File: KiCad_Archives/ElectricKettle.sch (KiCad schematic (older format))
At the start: 11 parts

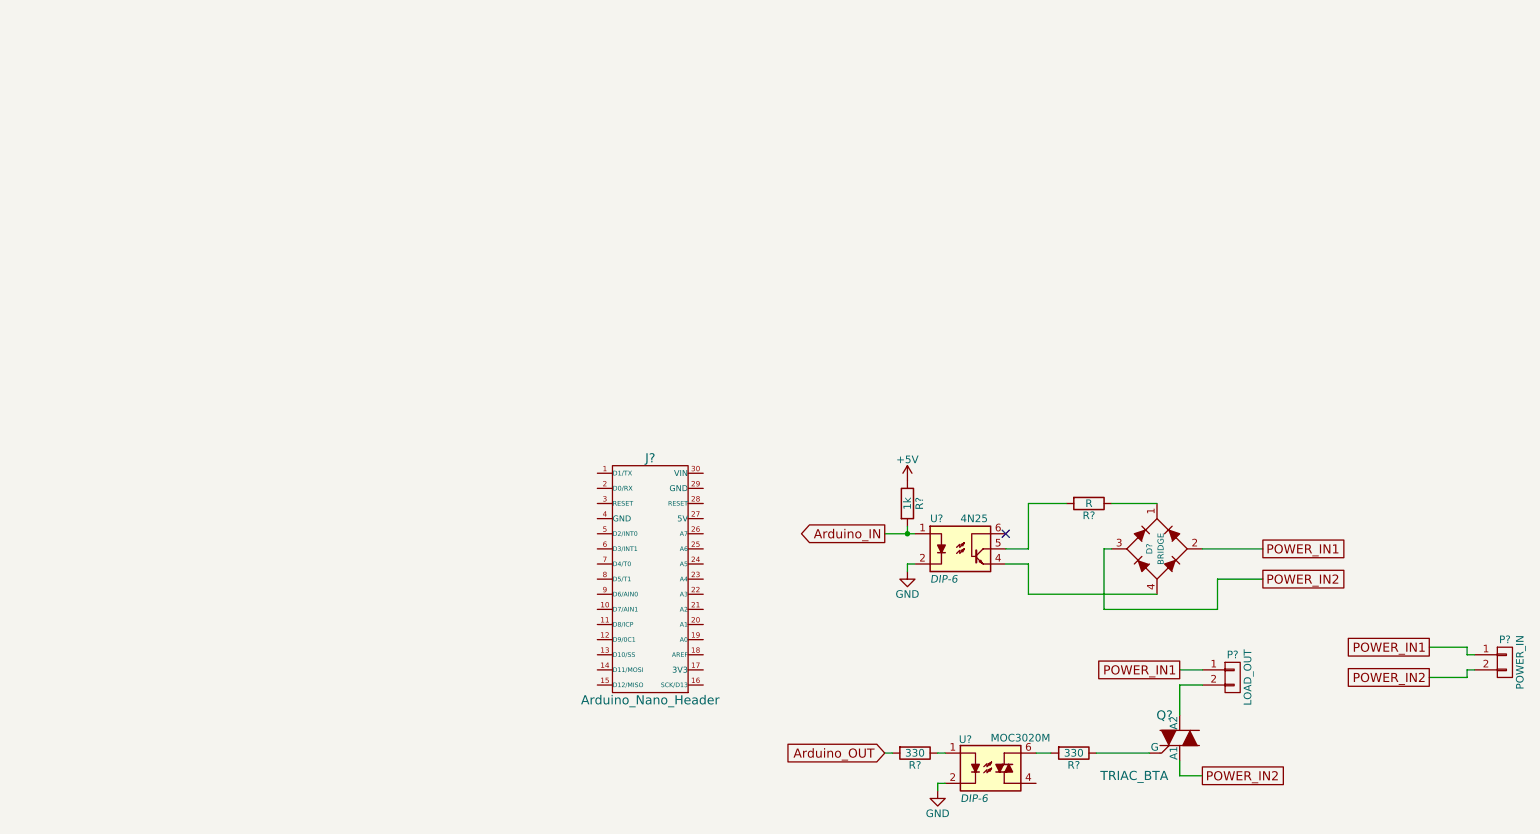
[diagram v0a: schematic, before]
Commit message: Complete Schematic V0.1
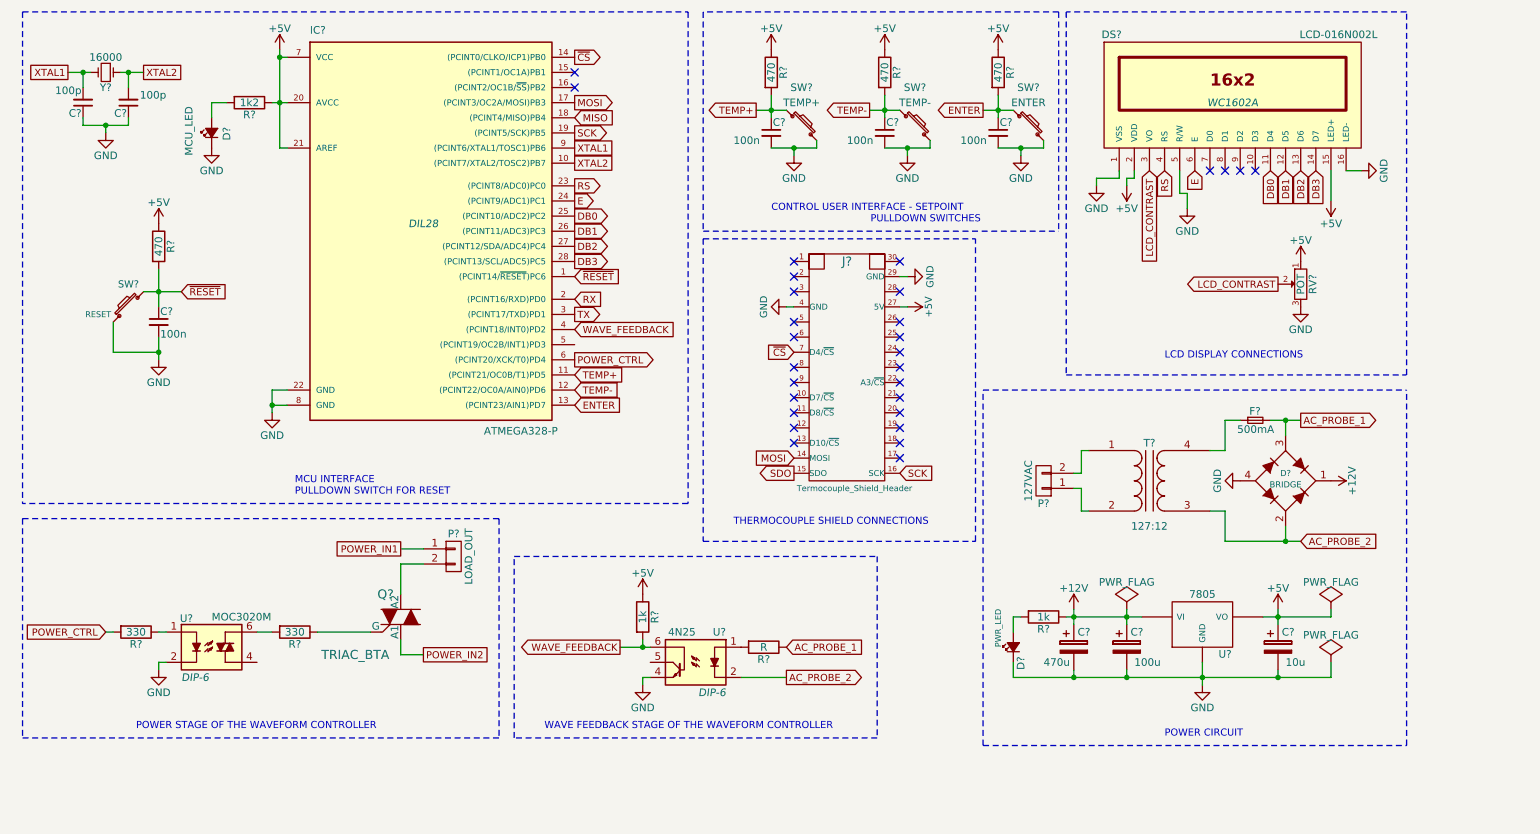
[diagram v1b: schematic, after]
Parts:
- removed J?: Arduino_Nano_Header, symbol Arduino_Nano_Header
- added C? (x2): 100p, symbol C_Small
- added C? (x4): 100n, symbol C_Small
- added C?: 470u, symbol CP
- added C?: 100u, symbol CP
- added C?: 10u, symbol CP
- added D?: MCU_LED, symbol Led_Small
- added D?: PWR_LED, symbol Led_Small
- added DS?: LCD-016N002L, WC1602A, symbol LCD-016N002L
- added F?: 500mA, symbol F_Small
- added IC?: ATMEGA328-P, DIL28, symbol ATMEGA328-P
- added J?: Termocouple_Shield_Header, symbol Termopar_Shield_Header
- added R?: 1k2, symbol R
- added R? (x4): 470, symbol R
- added R?: 1k, symbol R
- added RV?: POT, symbol POT
- added SW?: RESET, symbol SW_PUSH_SMALL
- added SW?: TEMP+, symbol SW_PUSH_SMALL
- added SW?: TEMP-, symbol SW_PUSH_SMALL
- added SW?: ENTER, symbol SW_PUSH_SMALL
- added T?: 127:12, symbol TRANSFO
- added U?: 7805, symbol 7805
- added Y?: 16000, symbol Crystal_Small
- P?: value POWER_IN -> 127VAC
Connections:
- net +5V: now also C?.1, DS?.15 (LED+), DS?.2 (VDD), IC?.20 (AVCC), IC?.21 (AREF), IC?.7 (VCC), J?.27 (5V), R?.1, R?.1, R?.1, R?.1, R?.1, RV?.1, U?.VO
- net GND: now also D?.4 (V-), U?.4, C?.1, C?.1, C?.2, C?.2, C?.2, C?.2, C?.2, C?.2, C?.2, D?.1 (K), D?.1 (K), DS?.1 (VSS), DS?.16 (LED-), DS?.5 (R/W), IC?.22 (GND), IC?.8 (GND), J?.29 (GND), J?.4 (GND), RV?.3, SW?.1, SW?.2, SW?.2, SW?.2, U?.GND; no longer U?.2
- net POWER_IN1: no longer D?.2 (~1), P?.1 (P1)
- net POWER_IN2: no longer D?.3 (~2), P?.2 (P2)
- net at R?.2: now also U?.1; no longer U?.5
- net WAVE_FEEDBACK: now reaches U?.6
- net WAVE_FEEDBACK: now also R?.2, IC?.4 ((PCINT18/INT0)PD2)
- net +12V: now reaches D?.1 (V+)
- net +12V: now also C?.1, C?.1, R?.1, U?.VI; no longer R?.1
- removed net Arduino_IN: R?.2, U?.1
- net Arduino_OUT renamed POWER_CTRL
- net POWER_CTRL: now also IC?.6 ((PCINT20/XCK/T0)PD4)
- new net: P?.1 (P1), T?.2 (AB)
- new net: P?.2 (P2), T?.1 (AA)
- new net: D?.2 (A), R?.2 (x2)
- new net: F?.1, T?.4 (SB)
- new net AC_PROBE_1: D?.3 (~2), F?.2, R?.1
- new net AC_PROBE_2: D?.2 (~1), T?.3 (SA), U?.2
- new net DB0: DS?.11 (D4), IC?.25 ((PCINT10/ADC2)PC2)
- new net DB1: DS?.12 (D5), IC?.26 ((PCINT11/ADC3)PC3)
- new net DB2: DS?.13 (D6), IC?.27 ((PCINT12/SDA/ADC4)PC4)
- new net DB3: DS?.14 (D7), IC?.28 ((PCINT13/SCL/ADC5)PC5)
- new net E: DS?.6 (E), IC?.24 ((PCINT9/ADC1)PC1)
- new net ENTER: C?.1, IC?.13 ((PCINT23/AIN1)PD7), R?.2, SW?.1
- new net LCD_CONTRAST: DS?.3 (VO), RV?.2
- new net MISO: IC?.18 ((PCINT4/MISO)PB4)
- new net MOSI: IC?.17 ((PCINT3/OC2A/MOSI)PB3), J?.14 (MOSI)
- new net RS: DS?.4 (RS), IC?.23 ((PCINT8/ADC0)PC0)
- new net RX: IC?.2 ((PCINT16/RXD)PD0)
- new net SCK: IC?.19 ((PCINT5/SCK)PB5), J?.16 (SCK)
- new net SDO: J?.15 (SDO)
- new net TEMP+: C?.1, IC?.11 ((PCINT21/OC0B/T1)PD5), R?.2, SW?.1
- new net TEMP-: C?.1, IC?.12 ((PCINT22/OC0A/AIN0)PD6), R?.2, SW?.1
- new net TX: IC?.3 ((PCINT17/TXD)PD1)
- new net XTAL1: C?.2, IC?.9 ((PCINT6/XTAL1/TOSC1)PB6), Y?.2
- new net XTAL2: C?.2, IC?.10 ((PCINT7/XTAL2/TOSC2)PB7), Y?.1
- new net ~CS: IC?.14 ((PCINT0/CLKO/ICP1)PB0), J?.7 (D4/~CS)
- new net ~RESET: C?.1, IC?.1 ((PCINT14/~RESET~)PC6), R?.2, SW?.2
- no-connect marks 1 -> 29
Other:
- note added: "CONTROL USER INTERFACE - SETPOINT\n PULLDOWN SWITCHES"
- note added: "LCD DISPLAY CONNECTIONS"
- note added: "MCU INTERFACE\nPULLDOWN SWITCH FOR RESET"
- note added: "POWER CIRCUIT\n"
- note added: "POWER STAGE OF THE WAVEFORM CONTROLLER"
- note added: "THERMOCOUPLE SHIELD CONNECTIONS\n"
- note added: "WAVE FEEDBACK STAGE OF THE WAVEFORM CONTROLLER\n"
- moved on the sheet: D?, P?, Q?, R?, U?
